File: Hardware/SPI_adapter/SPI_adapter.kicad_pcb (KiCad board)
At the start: 4 copper layers, 99.5 x 34.5 mm, 6 parts, among them J1 Conn_02x07_Top_Bottom, J2 Conn_Coaxial, U1 RF-LORA-868-SO

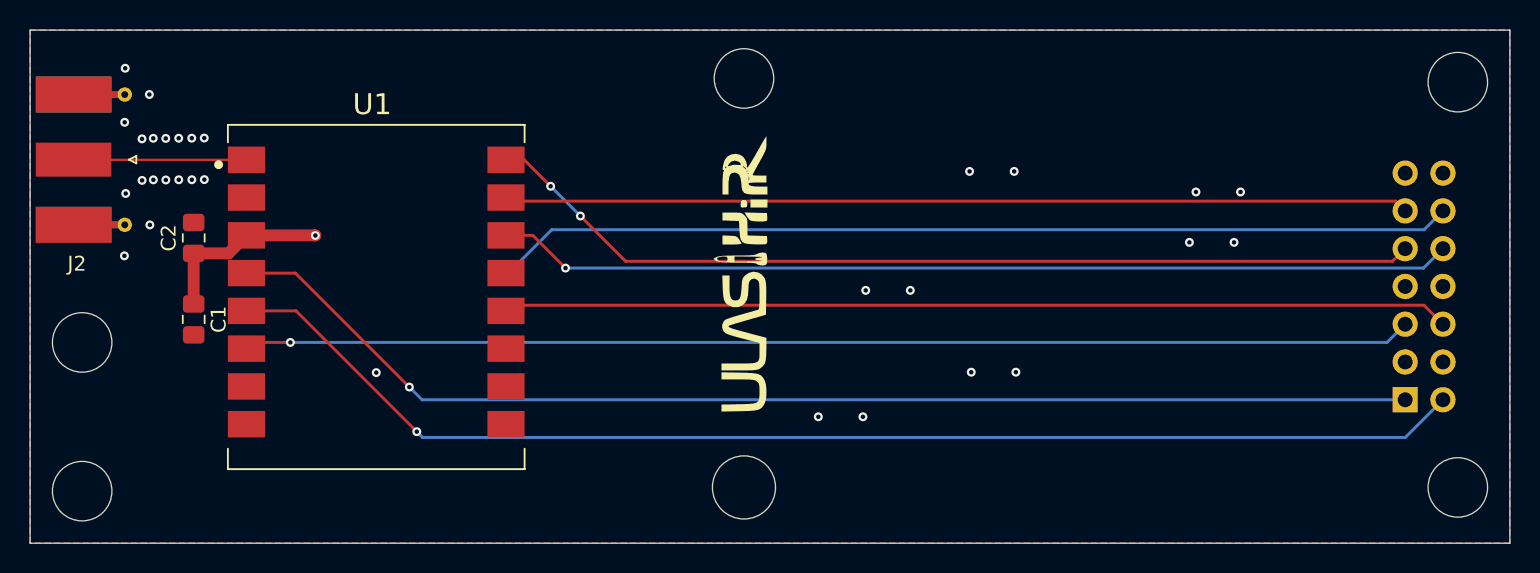
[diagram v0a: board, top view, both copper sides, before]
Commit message: hardware done
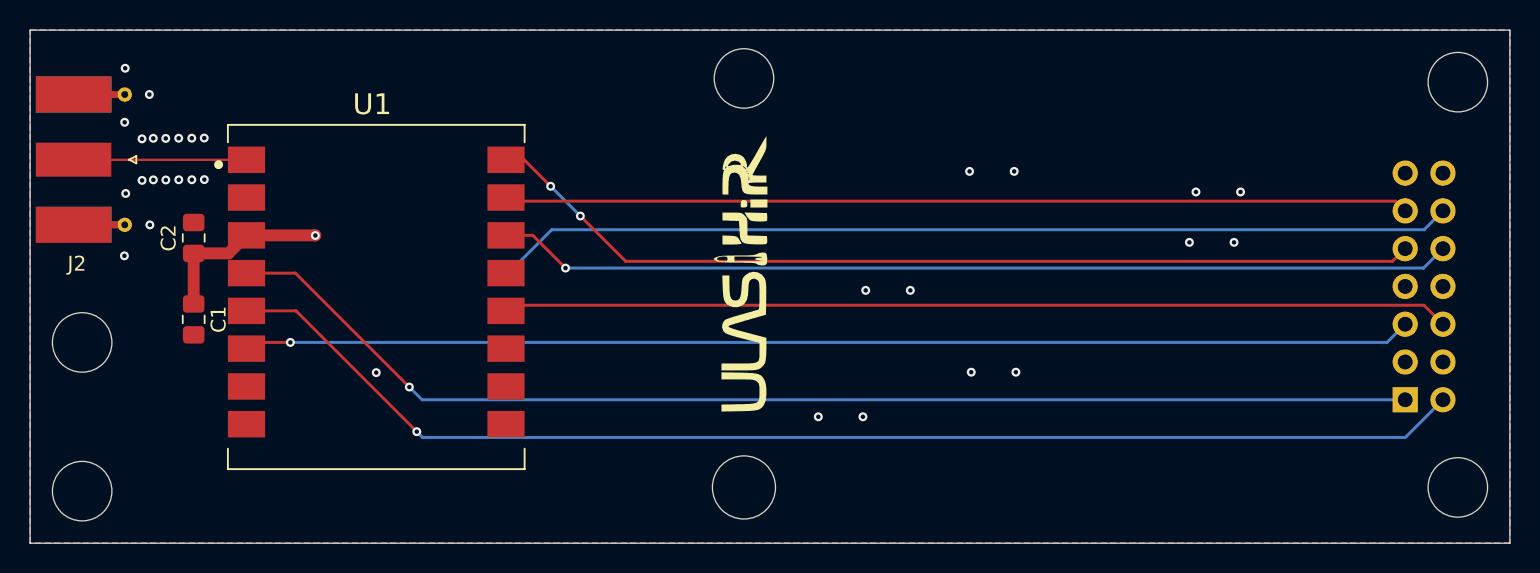
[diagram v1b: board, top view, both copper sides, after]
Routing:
- added copper zone on In2.Cu, net GND
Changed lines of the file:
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@@
 			(drillshape 0)
 			(scaleselection 1)
-			(outputdirectory "../Manufacturing/SPI_adapter/Gerber Output/")
+			(outputdirectory "../Manufacturing/SPI_adapter/fabrication/")
 		)
 	)
@@
 		(net 2)
 		(net_name "GND")
-		(layer "F.Cu")
+		(layers "F.Cu" "B.Cu" "In1.Cu" "In2.Cu")
 		(hatch edge 0.5)
 		(priority 2)
